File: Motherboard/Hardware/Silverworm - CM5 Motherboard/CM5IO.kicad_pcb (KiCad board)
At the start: 4 copper layers, 190 x 90 mm, 91 parts, among them J1 USB_C_Receptacle_USB2.0, J10 Conn_01x03, J11 THD-20-R, J12 Microfit 3-pin, J13 THD-02-R, J14 Microfit 6-pin, J15 Microfit 2-Pin, J16 Microfit 2-Pin, J17 Microfit 2-Pin, J18 Microfit 2-Pin, J2 Conn_01x22_Female, J20 USB_A, J23 Mega-Fit-1row-2pin, J24 Mega-Fit-2row-2pin, J3 Conn_01x22_Female, J4 THD-02-R, J5 USB3_A, J6 690-019-298-412, J7 690-019-298-412, J8 Conn_02x07_Odd_Even, J9 JST_SHBM04B-SRSS-TB, SW1 Right angle Tact button, U1 AP22653W6, U10 10uH, U2 RT9742SNGV, U3 TPD4EUSB30, U4 TPD4EUSB30, U5 MagJack-A70-112-331N126, U8 TPS54560DDAR, U9 SS54

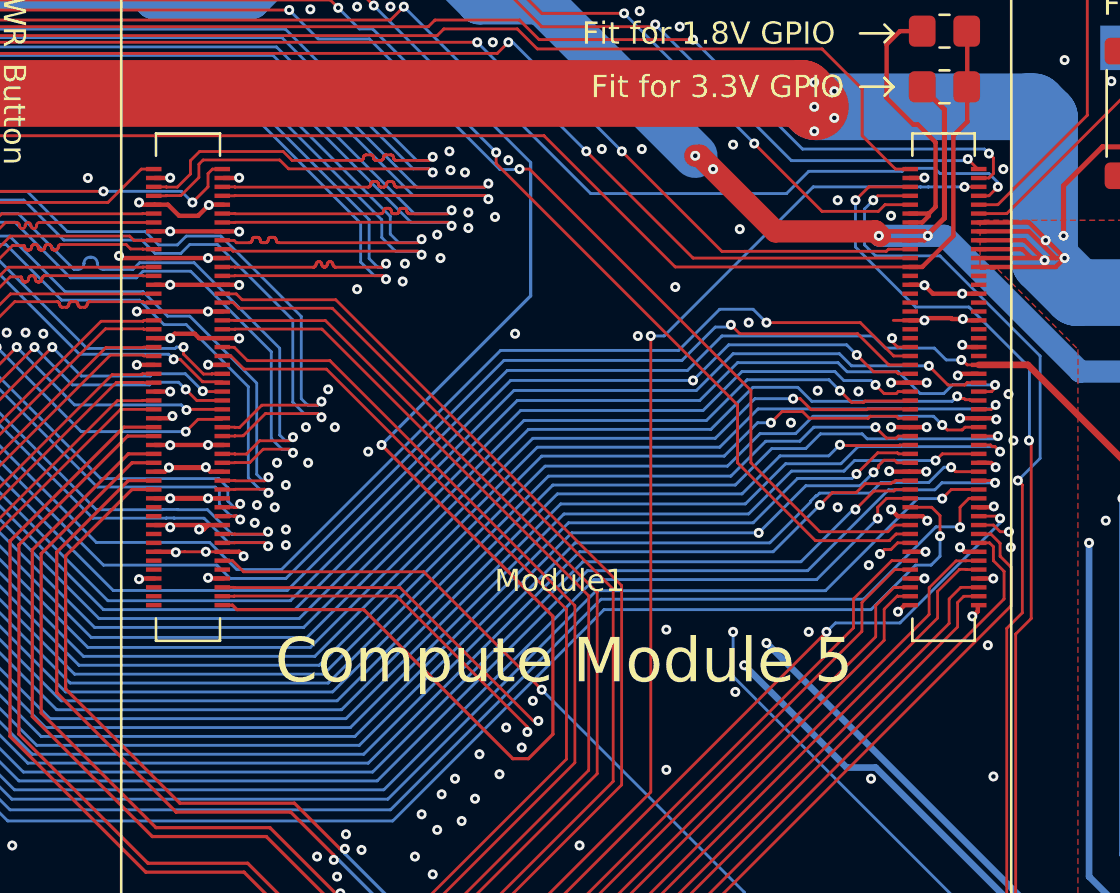
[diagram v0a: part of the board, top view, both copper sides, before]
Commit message: pcb aaaaaaah
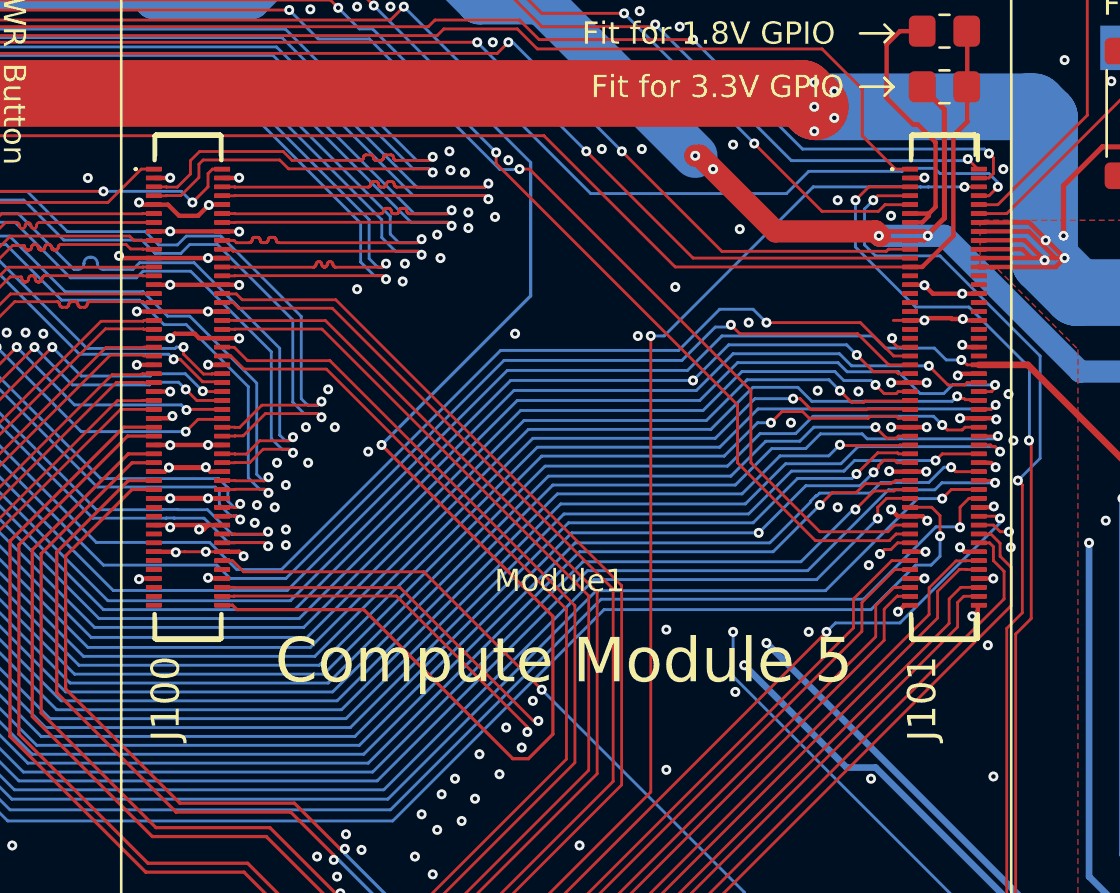
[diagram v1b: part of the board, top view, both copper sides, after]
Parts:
- added J100: 101642271001A1RLF, Amphenol 10164227-1001A1RLF:101642271001A1RLF, F.Cu at (165.5, 94.7)
- added J101: 101642271001A1RLF, Amphenol 10164227-1001A1RLF:101642271001A1RLF, F.Cu at (199.5, 94.7)
